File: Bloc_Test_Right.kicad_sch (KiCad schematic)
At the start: 44 parts, among them Q29 2N7000, Q30 2N7000, Q31 2N7000, Q32 2N7000, Q33 2N7000, Q34 2N7000

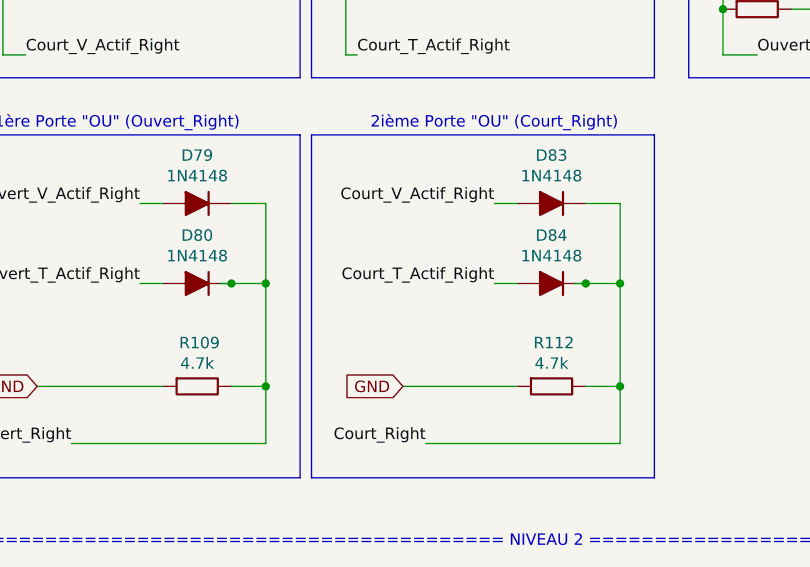
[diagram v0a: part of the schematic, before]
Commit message: Add files via upload
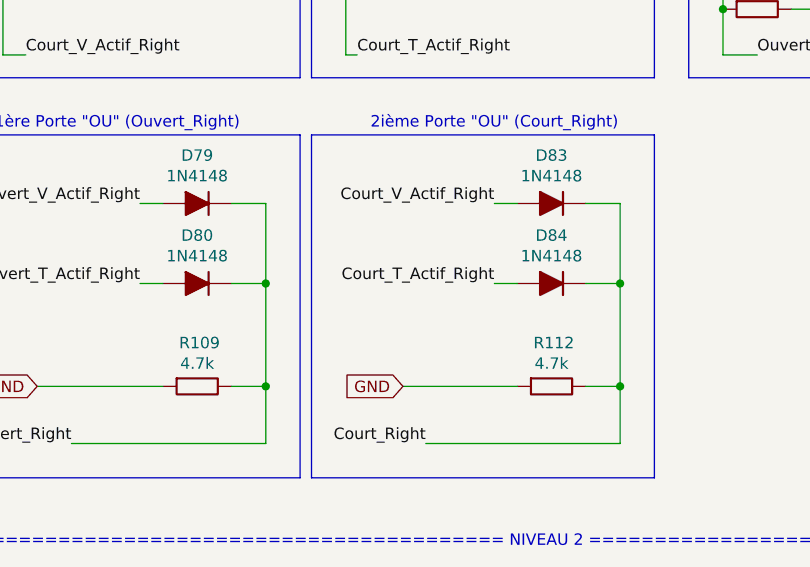
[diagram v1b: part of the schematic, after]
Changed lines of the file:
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@@
-	)
-	(junction
-		(at 91.44 86.36)
-		(diameter 0)
-		(color 0 0 0 0)
 	)
 	(junction
@@
 	)
 	(junction
-		(at 52.07 86.36)
-		(diameter 0)
-		(color 0 0 0 0)
-	)
-	(junction
 		(at 64.77 53.34)
 		(diameter 0)
@@
 	(wire
 		(pts
-			(xy 50.8 86.36) (xy 52.07 86.36)
-		)
-		(stroke
-			(width 0)
-			(type default)
-		)
-	)
-	(wire
-		(pts
 			(xy 156.21 50.8) (xy 162.56 50.8)
 		)
@@
 		)
 		(stroke
-			(width 0)
-			(type default)
-		)
-	)
-	(wire
-		(pts
-			(xy 90.17 86.36) (xy 91.44 86.36)
-		)
-		(stroke
